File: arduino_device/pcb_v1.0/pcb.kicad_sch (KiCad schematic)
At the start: 3 parts, among them SW1 SW_Push

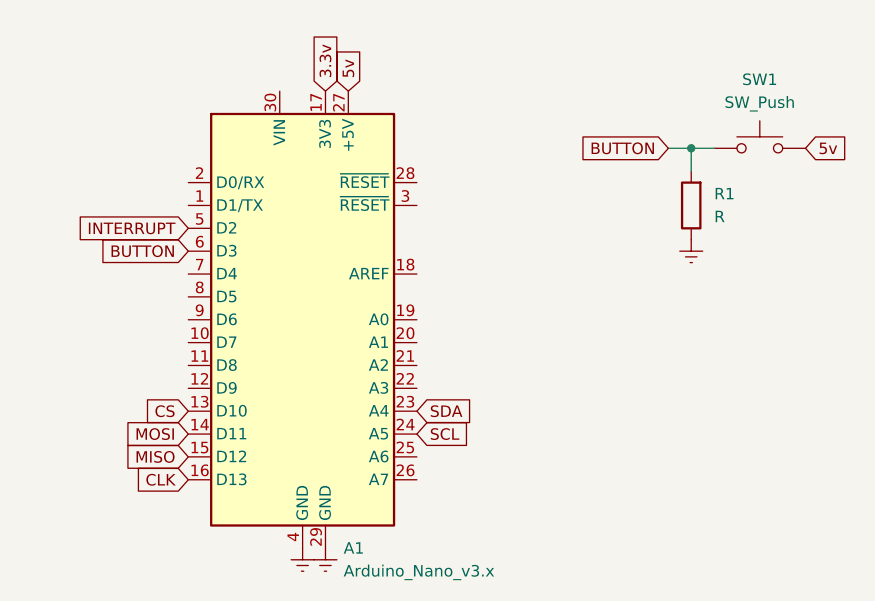
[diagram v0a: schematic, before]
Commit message: PCB v2.0
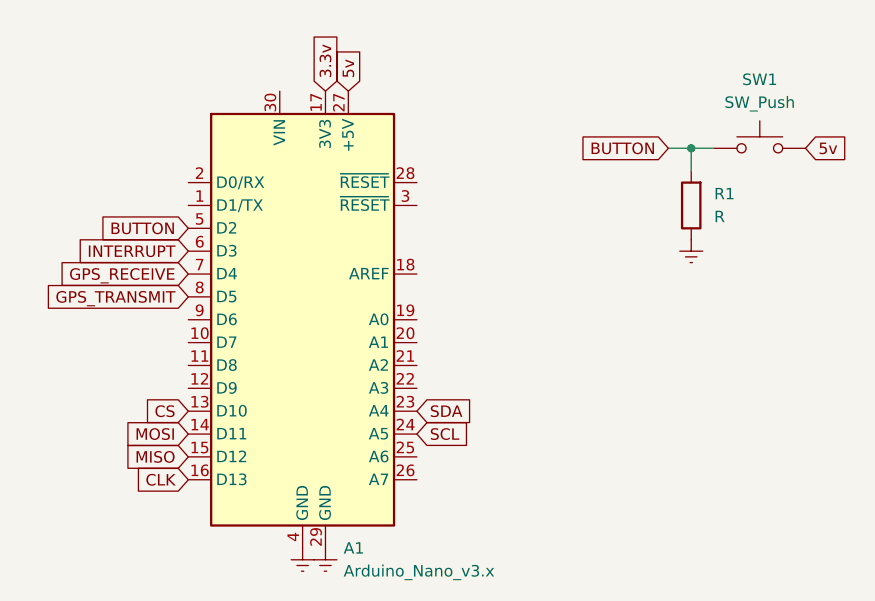
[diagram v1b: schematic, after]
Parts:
- SW1: footprint Connector_PinHeader_2.54mm:PinHeader_1x02_P2.54mm_Vertical -> TestPoint:TestPoint_Bridge_Pitch5.08mm_Drill0.7mm
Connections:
- net BUTTON: now also A1.5 (D2); no longer A1.6 (D3)
- net INTERRUPT: now also A1.6 (D3); no longer A1.5 (D2)
- net GPS_RECEIVE: now reaches A1.7 (D4)
- net GPS_TRANSMIT: now reaches A1.8 (D5)
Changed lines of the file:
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@@
     (stroke (width 0) (type default) (color 0 0 0 0))
   )
-  (global_label "INTERRUPT" (shape input) (at 119.38 81.28 180) (fields_autoplaced)
-    (effects (font (size 1.27 1.27)) (justify right))
-    (property "Intersheet References" "${INTERSHEET_REFS}" (id 0) (at 106.8069 81.2006 0)
-      (effects (font (size 1.27 1.27)) (justify right) hide)
-    )
-  )
   (global_label "3.3v" (shape input) (at 134.62 66.04 90) (fields_autoplaced)
     (effects (font (size 1.27 1.27)) (justify left))
@@
     )
   )
+  (global_label "GPS_TRANSMIT" (shape input) (at 119.38 88.9 180) (fields_autoplaced)
+    (effects (font (size 1.27 1.27)) (justify right))
+    (property "Intersheet References" "${INTERSHEET_REFS}" (id 0) (at 103.3598 88.8206 0)
+      (effects (font (size 1.27 1.27)) (justify right) hide)
+    )
+  )
   (global_label "CLK" (shape input) (at 119.38 109.22 180) (fields_autoplaced)
     (effects (font (size 1.27 1.27)) (justify right))
@@
     )
   )
+  (global_label "GPS_RECEIVE" (shape input) (at 119.38 86.36 180) (fields_autoplaced)
+    (effects (font (size 1.27 1.27)) (justify right))
+    (property "Intersheet References" "${INTERSHEET_REFS}" (id 0) (at 104.5693 86.2806 0)
+      (effects (font (size 1.27 1.27)) (justify right) hide)
+    )
+  )
   (global_label "SCL" (shape input) (at 144.78 104.14 0) (fields_autoplaced)
     (effects (font (size 1.27 1.27)) (justify left))
@@
     )
   )
+  (global_label "INTERRUPT" (shape input) (at 119.38 83.82 180) (fields_autoplaced)
+    (effects (font (size 1.27 1.27)) (justify right))
+    (property "Intersheet References" "${INTERSHEET_REFS}" (id 0) (at 106.8069 83.7406 0)
+      (effects (font (size 1.27 1.27)) (justify right) hide)
+    )
+  )
+  (global_label "BUTTON" (shape input) (at 119.38 81.28 180) (fields_autoplaced)
+    (effects (font (size 1.27 1.27)) (justify right))
+    (property "Intersheet References" "${INTERSHEET_REFS}" (id 0) (at 109.7702 81.2006 0)
+      (effects (font (size 1.27 1.27)) (justify right) hide)
+    )
+  )
   (global_label "5v" (shape input) (at 187.96 72.39 0) (fields_autoplaced)
     (effects (font (size 1.27 1.27)) (justify left))
     (property "Intersheet References" "${INTERSHEET_REFS}" (id 0) (at 192.5502 72.3106 0)
       (effects (font (size 1.27 1.27)) (justify left) hide)
-    )
-  )
-  (global_label "BUTTON" (shape input) (at 119.38 83.82 180) (fields_autoplaced)
-    (effects (font (size 1.27 1.27)) (justify right))
-    (property "Intersheet References" "${INTERSHEET_REFS}" (id 0) (at 109.7702 83.7406 0)
-      (effects (font (size 1.27 1.27)) (justify right) hide)
     )
   )
@@
     (property "Reference" "SW1" (id 0) (at 182.88 64.77 0))
     (property "Value" "SW_Push" (id 1) (at 182.88 67.31 0))
-    (property "Footprint" "Connector_PinHeader_2.54mm:PinHeader_1x02_P2.54mm_Vertical" (id 2) (at 182.88 67.31 0)
+    (property "Footprint" "TestPoint:TestPoint_Bridge_Pitch5.08mm_Drill0.7mm" (id 2) (at 182.88 67.31 0)
       (effects (font (size 1.27 1.27)) hide)
     )
@@
     )
     (path "/3111f524-7522-420c-b2f5-77c2e5bfff6c"
-      (reference "SW1") (unit 1) (value "SW_Push") (footprint "Connector_PinHeader_2.54mm:PinHeader_1x02_P2.54mm_Vertical")
-    )
-  )
+      (reference "SW1") (unit 1) (value "SW_Push") (footprint "TestPoint:TestPoint_Bridge_Pitch5.08mm_Drill0.7mm")
+    )
+  )
